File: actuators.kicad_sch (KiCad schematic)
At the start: 4 parts, among them J20 09564527612

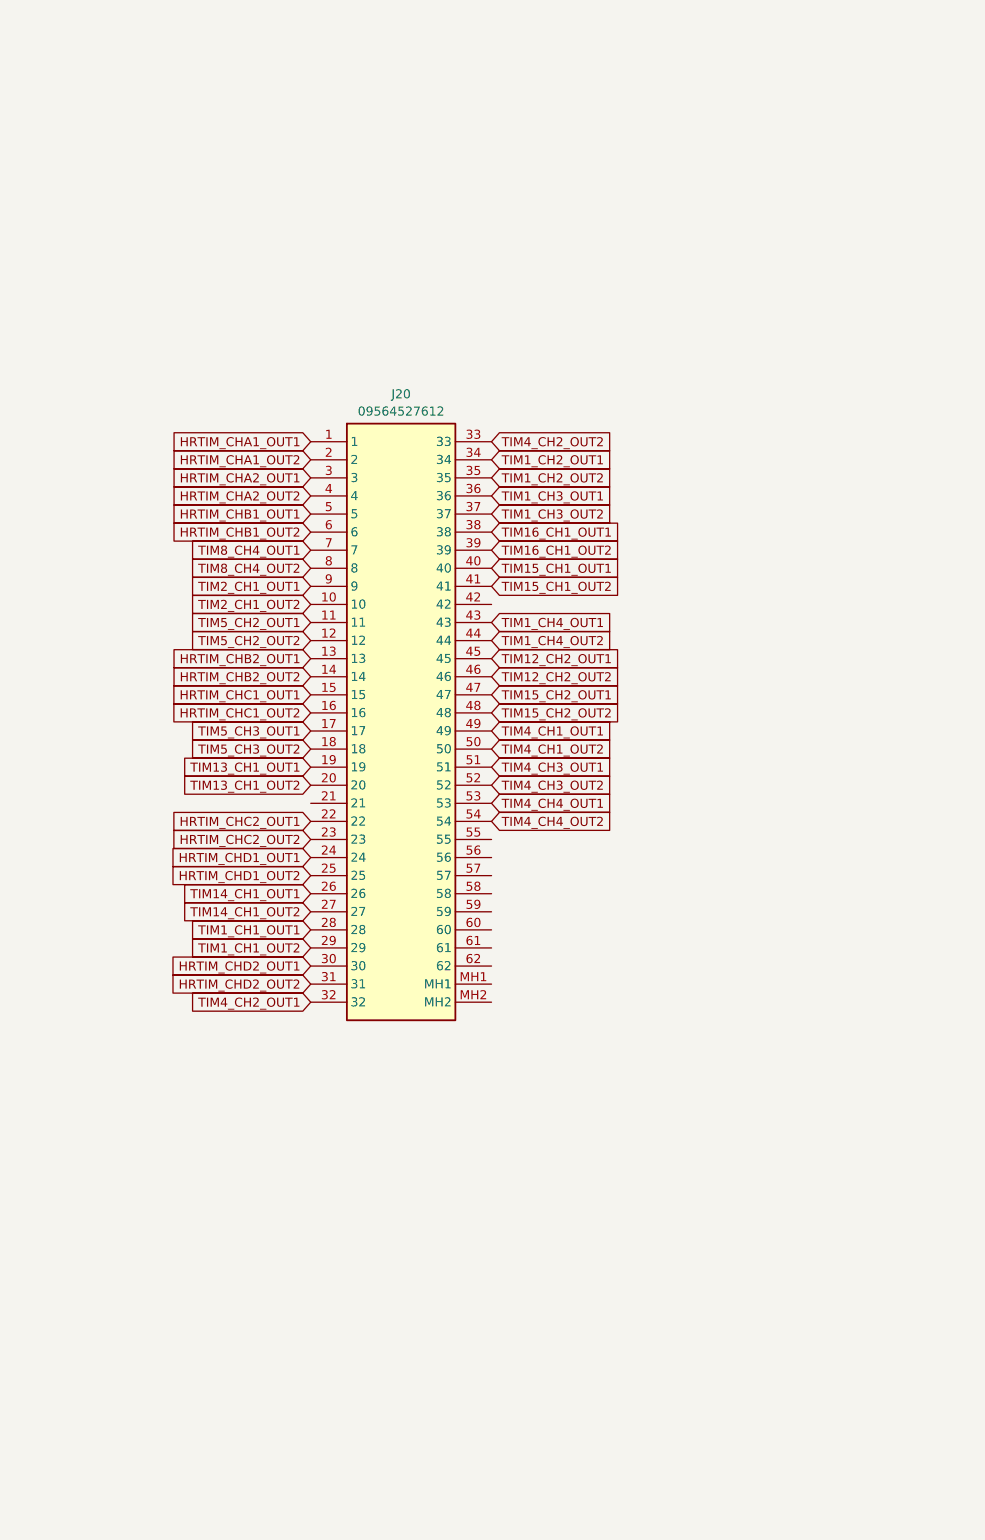
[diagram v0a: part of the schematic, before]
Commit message: Add files via upload
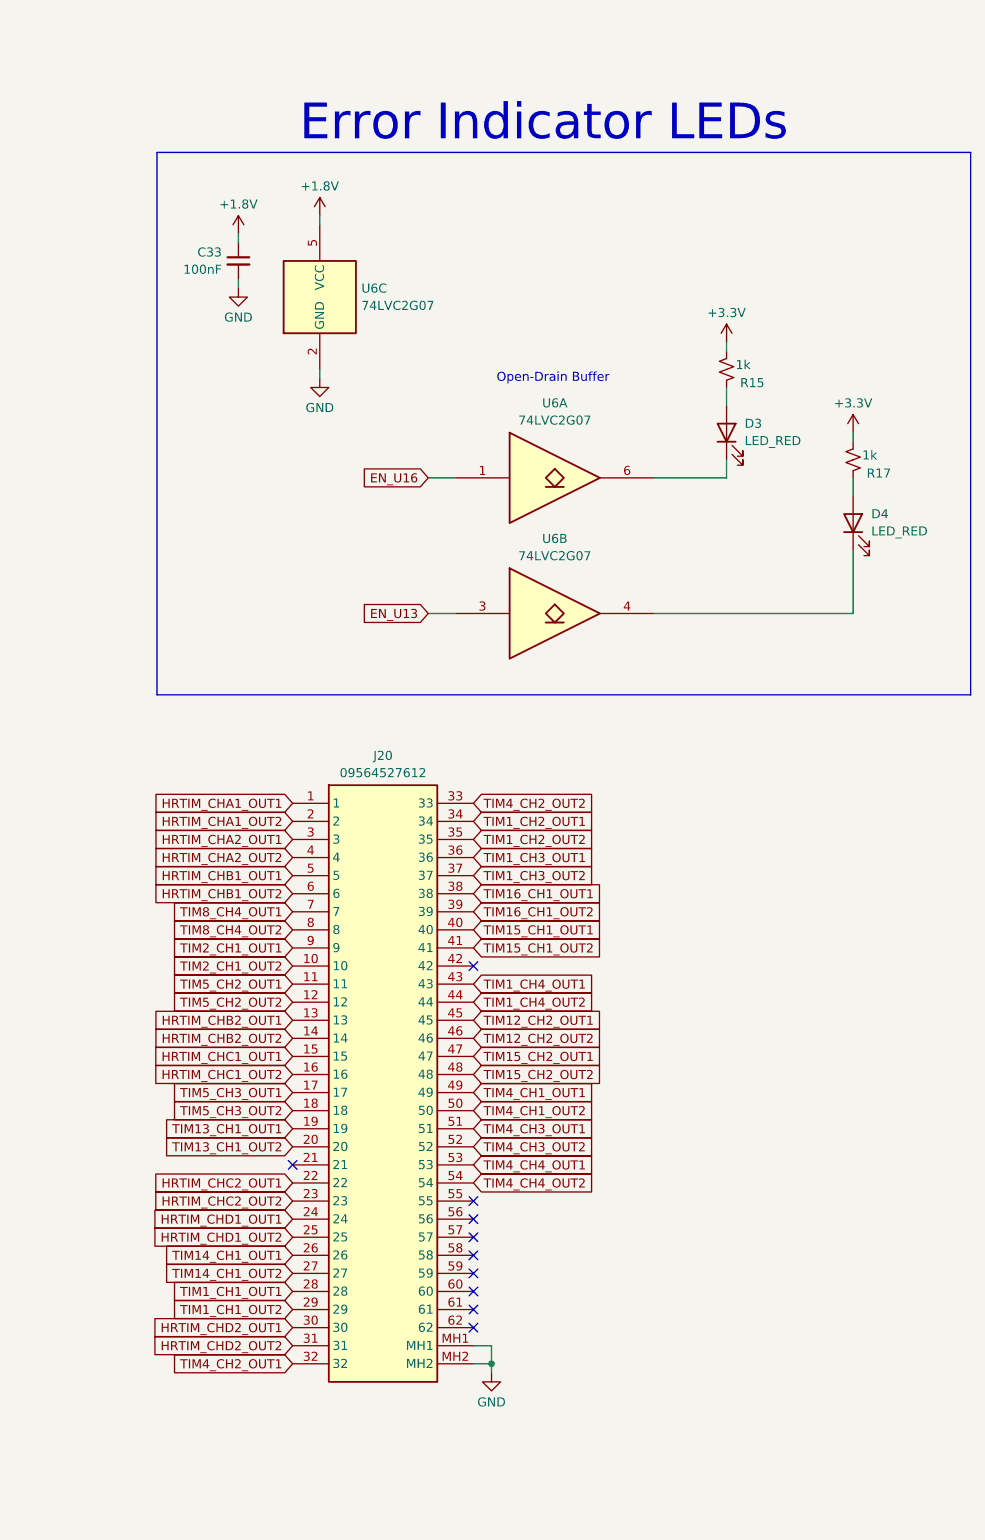
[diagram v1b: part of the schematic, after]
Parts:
- added C33: 100nF, Capacitor_SMD:C_0402_1005Metric, symbol Device:C_Small
- added D3, D4: LED_RED, LED_SMD:LED_0603_1608Metric, symbol Device:LED
- added R15, R17: 1k, Resistor_SMD:R_0402_1005Metric, symbol Device:R_Small_US
- added U6: 74LVC2G07, Package_TO_SOT_SMD:SOT-23-6, symbol 74xGxx:74LVC2G07
- J20: footprint 09564527612 -> components_2:09564527612
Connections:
- net +1.8V: now also C33.1, U6.5 (VCC)
- net GND: now also J20.MH1, J20.MH2, C33.2, U6.2 (GND)
- new net: D4.2 (A), R17.2
- new net: D4.1 (K), U6.4
- new net: D3.1 (K), U6.6
- new net: D3.2 (A), R15.2
- new net +3.3V: R15.1, R17.1
- new net EN_U13: U6.3
- new net EN_U16: U6.1
- no-connect marks 0 -> 10
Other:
- note added: "Error Indicator LEDs"
- note added: "Open-Drain Buffer"
- moved on the sheet: J20
